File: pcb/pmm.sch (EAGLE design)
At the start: 25 parts, among them IC3 STM32F042F4, SW3 324_SW, SW4 324_SW, U2 USBC_16P, U4 XC6206_DEV

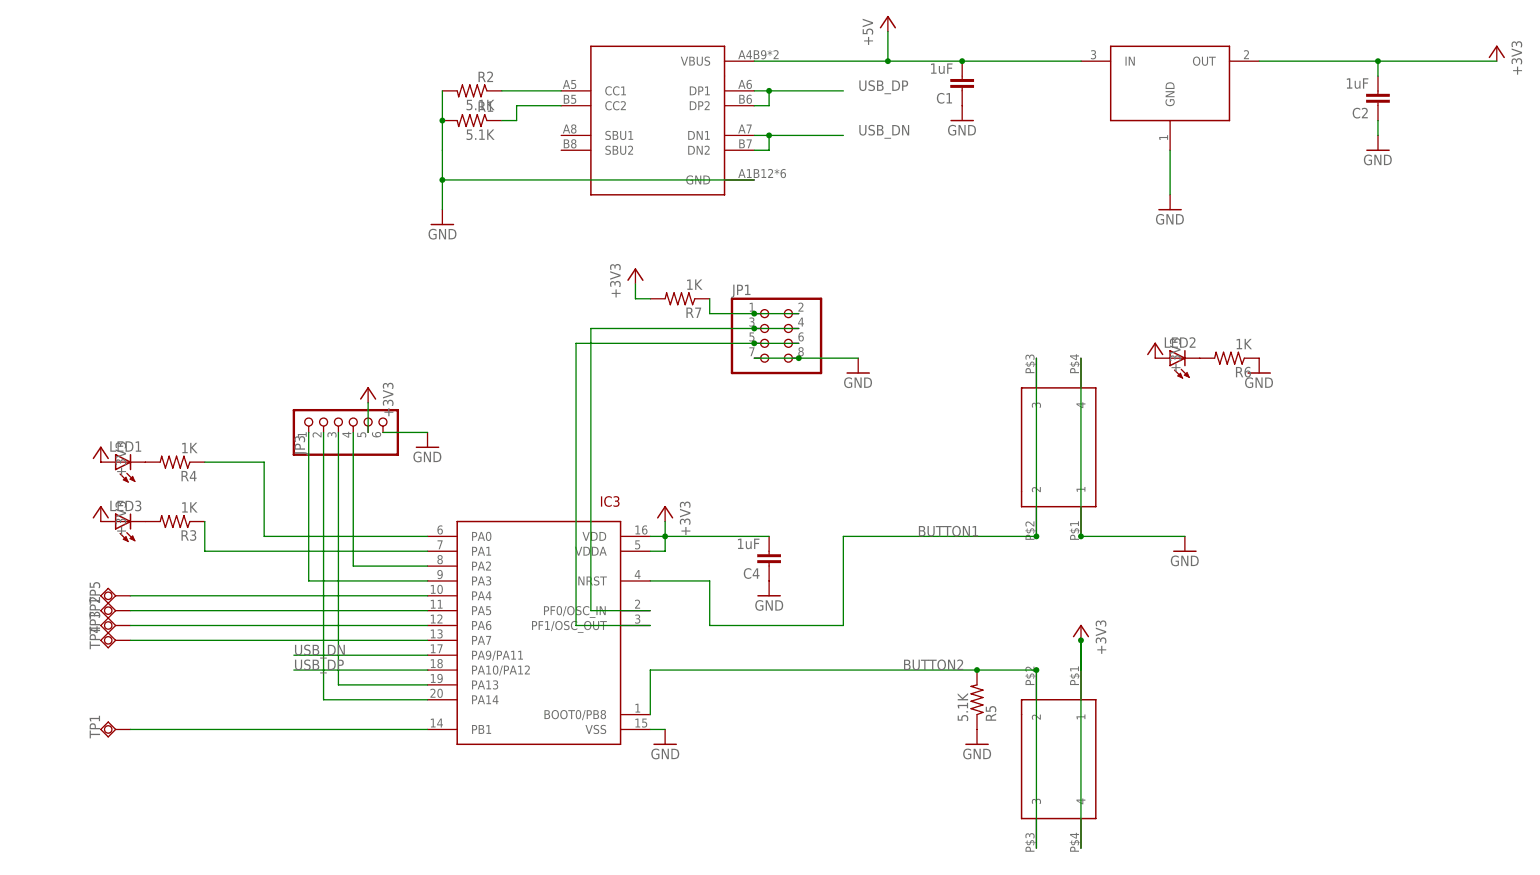
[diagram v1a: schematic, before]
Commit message: updated pcb for next production run
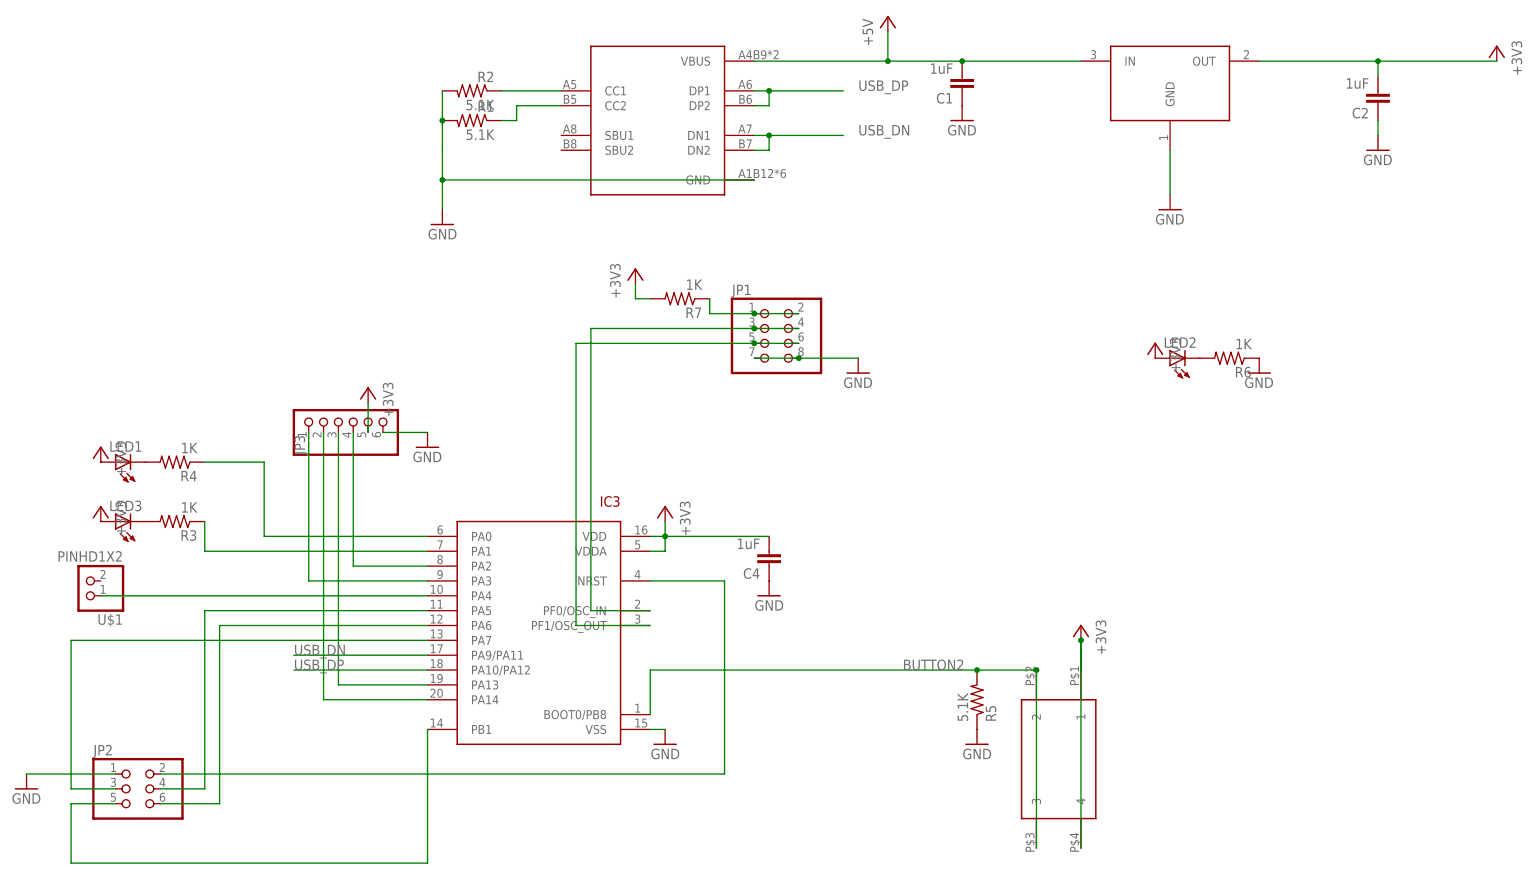
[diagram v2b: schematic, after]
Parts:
- removed SW3: 324_SW, 3pos_slide_switch_centered:324_SW
- removed TP1, TP2, TP3, TP4, TP5: TPSQTP10SQ, testpad:TPSQTP10SQ
- added JP2: (no value), pinhead:PINHD-2X3
- added U$1: PINHD1X2, adafruit_changed:PINHD1X2
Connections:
- removed net BUTTON1: IC3.NRST, SW3.2, SW3.3
- new net N$16: IC3.PA4, U$1.1
- net GND: now also JP2.1; no longer SW3.1, SW3.4
- net N$11: now also IC3.PA5, JP2.4; no longer IC3.PA7, TP4.TP
- net N$12: now also JP2.6; no longer TP3.TP
- net N$13: now also IC3.PA7, JP2.3; no longer IC3.PA5, TP2.TP
- net N$14: now also JP2.5; no longer TP1.TP
- net N$15: now also IC3.NRST, JP2.2; no longer IC3.PA4, TP5.TP
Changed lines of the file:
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@@
 <?xml version="1.0" encoding="utf-8"?>
 <!DOCTYPE eagle SYSTEM "eagle.dtd">
-<eagle version="9.6.1">
+<eagle version="9.6.2">
 <drawing>
 <settings>
@@
 <part name="GND8" library="supply1" deviceset="GND" device=""/>
 <part name="GND11" library="supply1" library_urn="urn:adsk.eagle:library:371" deviceset="GND" device=""/>
-<part name="SW3" library="3pos_slide_switch_centered" deviceset="324_SW" device="" value="324_SW"/>
 <part name="SW4" library="3pos_slide_switch_centered" deviceset="324_SW" device="" value="324_SW"/>
 <part name="LED1" library="adafruit" deviceset="LED" device="CHIP-LED0805"/>
@@
 <part name="GND3" library="backplane" deviceset="GND" device=""/>
 <part name="R7" library="SparkFun-Passives" deviceset="RESISTOR" device="0805-RES" value="1K"/>
-<part name="TP1" library="testpad" library_urn="urn:adsk.eagle:library:385" deviceset="TPSQ" device="TP10SQ" package3d_urn="urn:adsk.eagle:package:27962/1" value="TPSQTP10SQ"/>
-<part name="TP2" library="testpad" library_urn="urn:adsk.eagle:library:385" deviceset="TPSQ" device="TP10SQ" package3d_urn="urn:adsk.eagle:package:27962/1" value="TPSQTP10SQ"/>
-<part name="TP3" library="testpad" library_urn="urn:adsk.eagle:library:385" deviceset="TPSQ" device="TP10SQ" package3d_urn="urn:adsk.eagle:package:27962/1" value="TPSQTP10SQ"/>
-<part name="TP4" library="testpad" library_urn="urn:adsk.eagle:library:385" deviceset="TPSQ" device="TP10SQ" package3d_urn="urn:adsk.eagle:package:27962/1" value="TPSQTP10SQ"/>
-<part name="TP5" library="testpad" library_urn="urn:adsk.eagle:library:385" deviceset="TPSQ" device="TP10SQ" package3d_urn="urn:adsk.eagle:package:27962/1" value="TPSQTP10SQ"/>
+<part name="JP2" library="pinhead" library_urn="urn:adsk.eagle:library:325" deviceset="PINHD-2X3" device="" package3d_urn="urn:adsk.eagle:package:22462/2"/>
+<part name="U$1" library="adafruit_changed" deviceset="PINHD1X2" device=""/>
 </parts>
 <sheets>
@@
 <attribute name="VALUE" x="43.18" y="27.94" size="1.778" layer="96" rot="MR0"/>
 </instance>
-<instance part="GND11" gate="1" x="111.76" y="38.1" smashed="yes">
-<attribute name="VALUE" x="109.22" y="35.56" size="1.778" layer="96"/>
-</instance>
-<instance part="SW3" gate="G$1" x="91.44" y="55.88" smashed="yes" rot="R90"/>
+<instance part="GND11" gate="1" x="-86.36" y="-2.54" smashed="yes">
+<attribute name="VALUE" x="-88.9" y="-5.08" size="1.778" layer="96"/>
+</instance>
 <instance part="SW4" gate="G$1" x="91.44" y="2.54" smashed="yes" rot="MR270"/>
 <instance part="LED1" gate="G$1" x="-71.12" y="53.34" smashed="yes" rot="R90">
@@
 <attribute name="VALUE" x="29.21" y="84.582" size="1.778" layer="96" rot="R180"/>
 </instance>
-<instance part="TP1" gate="G$1" x="-71.12" y="7.62" smashed="yes" rot="R270">
-<attribute name="NAME" x="-75.565" y="10.16" size="1.778" layer="95" rot="R270"/>
-<attribute name="TP_SIGNAL_NAME" x="-72.39" y="5.08" size="1.778" layer="97" rot="R270"/>
-</instance>
-<instance part="TP2" gate="G$1" x="-71.12" y="27.94" smashed="yes" rot="R270">
-<attribute name="NAME" x="-75.565" y="30.48" size="1.778" layer="95" rot="R270"/>
-<attribute name="TP_SIGNAL_NAME" x="-72.39" y="25.4" size="1.778" layer="97" rot="R270"/>
-</instance>
-<instance part="TP3" gate="G$1" x="-71.12" y="25.4" smashed="yes" rot="R270">
-<attribute name="NAME" x="-75.565" y="27.94" size="1.778" layer="95" rot="R270"/>
-<attribute name="TP_SIGNAL_NAME" x="-72.39" y="22.86" size="1.778" layer="97" rot="R270"/>
-</instance>
-<instance part="TP4" gate="G$1" x="-71.12" y="22.86" smashed="yes" rot="R270">
-<attribute name="NAME" x="-75.565" y="25.4" size="1.778" layer="95" rot="R270"/>
-<attribute name="TP_SIGNAL_NAME" x="-72.39" y="20.32" size="1.778" layer="97" rot="R270"/>
-</instance>
-<instance part="TP5" gate="G$1" x="-71.12" y="30.48" smashed="yes" rot="R270">
-<attribute name="NAME" x="-75.565" y="33.02" size="1.778" layer="95" rot="R270"/>
-<attribute name="TP_SIGNAL_NAME" x="-72.39" y="27.94" size="1.778" layer="97" rot="R270"/>
+<instance part="JP2" gate="A" x="-68.58" y="-2.54" smashed="yes">
+<attribute name="NAME" x="-74.93" y="3.175" size="1.778" layer="95"/>
+<attribute name="VALUE" x="-74.93" y="-10.16" size="1.778" layer="96"/>
+</instance>
+<instance part="U$1" gate="1" x="-76.2" y="33.02" smashed="yes" rot="R180">
+<attribute name="NAME" x="-69.85" y="27.305" size="1.778" layer="95" rot="R180"/>
+<attribute name="VALUE" x="-69.85" y="38.1" size="1.778" layer="96" rot="R180"/>
 </instance>
 </instances>
@@
 </segment>
 <segment>
-<pinref part="GND11" gate="1" pin="GND"/>
-<pinref part="SW3" gate="G$1" pin="1"/>
-<wire x1="93.98" y1="40.64" x2="111.76" y2="40.64" width="0.1524" layer="91"/>
-<pinref part="SW3" gate="G$1" pin="4"/>
-<wire x1="93.98" y1="71.12" x2="93.98" y2="40.64" width="0.1524" layer="91"/>
-<junction x="93.98" y="40.64"/>
-</segment>
-<segment>
 <pinref part="R6" gate="G$1" pin="1"/>
 <pinref part="GND9" gate="1" pin="GND"/>
@@
 <pinref part="GND3" gate="1" pin="GND"/>
 <wire x1="-25.4" y1="58.42" x2="-17.78" y2="58.42" width="0.1524" layer="91"/>
+</segment>
+<segment>
+<pinref part="JP2" gate="A" pin="1"/>
+<pinref part="GND11" gate="1" pin="GND"/>
+<wire x1="-71.12" y1="0" x2="-86.36" y2="0" width="0.1524" layer="91"/>
 </segment>
 </net>
@@
 <junction x="60.96" y="121.92"/>
 <pinref part="U4" gate="G$1" pin="IN"/>
-</segment>
-</net>
-<net name="BUTTON1" class="0">
-<segment>
-<label x="66.04" y="40.64" size="1.778" layer="95"/>
-<pinref part="SW3" gate="G$1" pin="2"/>
-<wire x1="53.34" y1="40.64" x2="86.36" y2="40.64" width="0.1524" layer="91"/>
-<pinref part="SW3" gate="G$1" pin="3"/>
-<wire x1="86.36" y1="71.12" x2="86.36" y2="40.64" width="0.1524" layer="91"/>
-<junction x="86.36" y="40.64"/>
-<pinref part="IC3" gate="G$1" pin="NRST"/>
-<wire x1="20.32" y1="33.02" x2="30.48" y2="33.02" width="0.1524" layer="91"/>
-<wire x1="30.48" y1="33.02" x2="30.48" y2="25.4" width="0.1524" layer="91"/>
-<wire x1="30.48" y1="25.4" x2="53.34" y2="25.4" width="0.1524" layer="91"/>
-<wire x1="53.34" y1="25.4" x2="53.34" y2="40.64" width="0.1524" layer="91"/>
 </segment>
 </net>
@@
 <net name="N$11" class="0">
 <segment>
+<pinref part="IC3" gate="G$1" pin="PA5"/>
+<wire x1="-17.78" y1="27.94" x2="-55.88" y2="27.94" width="0.1524" layer="91"/>
+<wire x1="-55.88" y1="27.94" x2="-55.88" y2="-2.54" width="0.1524" layer="91"/>
+<pinref part="JP2" gate="A" pin="4"/>
+<wire x1="-55.88" y1="-2.54" x2="-63.5" y2="-2.54" width="0.1524" layer="91"/>
+</segment>
+</net>
+<net name="N$12" class="0">
+<segment>
+<pinref part="IC3" gate="G$1" pin="PA6"/>
+<wire x1="-17.78" y1="25.4" x2="-53.34" y2="25.4" width="0.1524" layer="91"/>
+<wire x1="-53.34" y1="25.4" x2="-53.34" y2="-5.08" width="0.1524" layer="91"/>
+<pinref part="JP2" gate="A" pin="6"/>
+<wire x1="-53.34" y1="-5.08" x2="-63.5" y2="-5.08" width="0.1524" layer="91"/>
+</segment>
+</net>
+<net name="N$13" class="0">
+<segment>
 <pinref part="IC3" gate="G$1" pin="PA7"/>
-<pinref part="TP4" gate="G$1" pin="TP"/>
-<wire x1="-17.78" y1="22.86" x2="-68.58" y2="22.86" width="0.1524" layer="91"/>
-</segment>
-</net>
-<net name="N$12" class="0">
-<segment>
-<pinref part="IC3" gate="G$1" pin="PA6"/>
-<pinref part="TP3" gate="G$1" pin="TP"/>
-<wire x1="-17.78" y1="25.4" x2="-68.58" y2="25.4" width="0.1524" layer="91"/>
-</segment>
-</net>
-<net name="N$13" class="0">
-<segment>
-<pinref part="IC3" gate="G$1" pin="PA5"/>
-<pinref part="TP2" gate="G$1" pin="TP"/>
-<wire x1="-17.78" y1="27.94" x2="-68.58" y2="27.94" width="0.1524" layer="91"/>
+<wire x1="-17.78" y1="22.86" x2="-78.74" y2="22.86" width="0.1524" layer="91"/>
+<wire x1="-78.74" y1="22.86" x2="-78.74" y2="-2.54" width="0.1524" layer="91"/>
+<pinref part="JP2" gate="A" pin="3"/>
+<wire x1="-78.74" y1="-2.54" x2="-71.12" y2="-2.54" width="0.1524" layer="91"/>
 </segment>
 </net>
@@
 <segment>
 <pinref part="IC3" gate="G$1" pin="PB1"/>
-<pinref part="TP1" gate="G$1" pin="TP"/>
-<wire x1="-68.58" y1="7.62" x2="-17.78" y2="7.62" width="0.1524" layer="91"/>
+<wire x1="-17.78" y1="7.62" x2="-17.78" y2="-15.24" width="0.1524" layer="91"/>
+<wire x1="-17.78" y1="-15.24" x2="-78.74" y2="-15.24" width="0.1524" layer="91"/>
+<wire x1="-78.74" y1="-15.24" x2="-78.74" y2="-5.08" width="0.1524" layer="91"/>
+<pinref part="JP2" gate="A" pin="5"/>
+<wire x1="-78.74" y1="-5.08" x2="-71.12" y2="-5.08" width="0.1524" layer="91"/>
 </segment>
 </net>
 <net name="N$15" class="0">
 <segment>
+<pinref part="IC3" gate="G$1" pin="NRST"/>
+<wire x1="20.32" y1="33.02" x2="33.02" y2="33.02" width="0.1524" layer="91"/>
+<wire x1="33.02" y1="33.02" x2="33.02" y2="0" width="0.1524" layer="91"/>
+<pinref part="JP2" gate="A" pin="2"/>
+<wire x1="33.02" y1="0" x2="-63.5" y2="0" width="0.1524" layer="91"/>
+</segment>
+</net>
+<net name="N$16" class="0">
+<segment>
 <pinref part="IC3" gate="G$1" pin="PA4"/>
-<pinref part="TP5" gate="G$1" pin="TP"/>
-<wire x1="-17.78" y1="30.48" x2="-68.58" y2="30.48" width="0.1524" layer="91"/>
-</segment>
-</net>
+<pinref part="U$1" gate="1" pin="1"/>
+<wire x1="-17.78" y1="30.48" x2="-73.66" y2="30.48" width="0.1524" layer="91"/>
+</segment>
+</net>
